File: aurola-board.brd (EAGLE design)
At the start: 86.4 x 31.8 mm, 84 parts, among them IC1 STM32F051C6T, J1 CONN_PWM, J2 CONN_TEMP, J3 CONN_FAN, J4 CONN_EC11, J5 CONN_I2C, P1 KF128-2P, Q1 600mA/40V, U1 ESP-01F, U2 BL9341, U3 BL9341

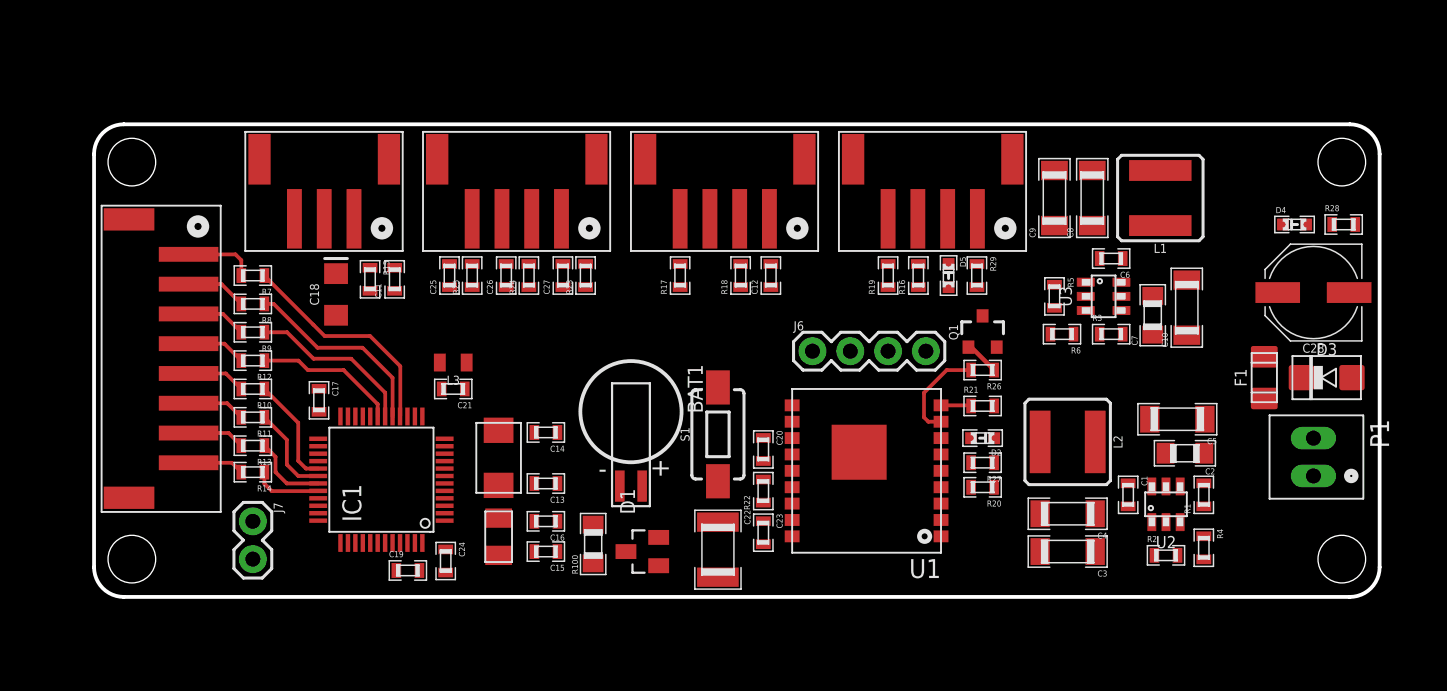
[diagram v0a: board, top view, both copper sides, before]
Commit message: 完成布局
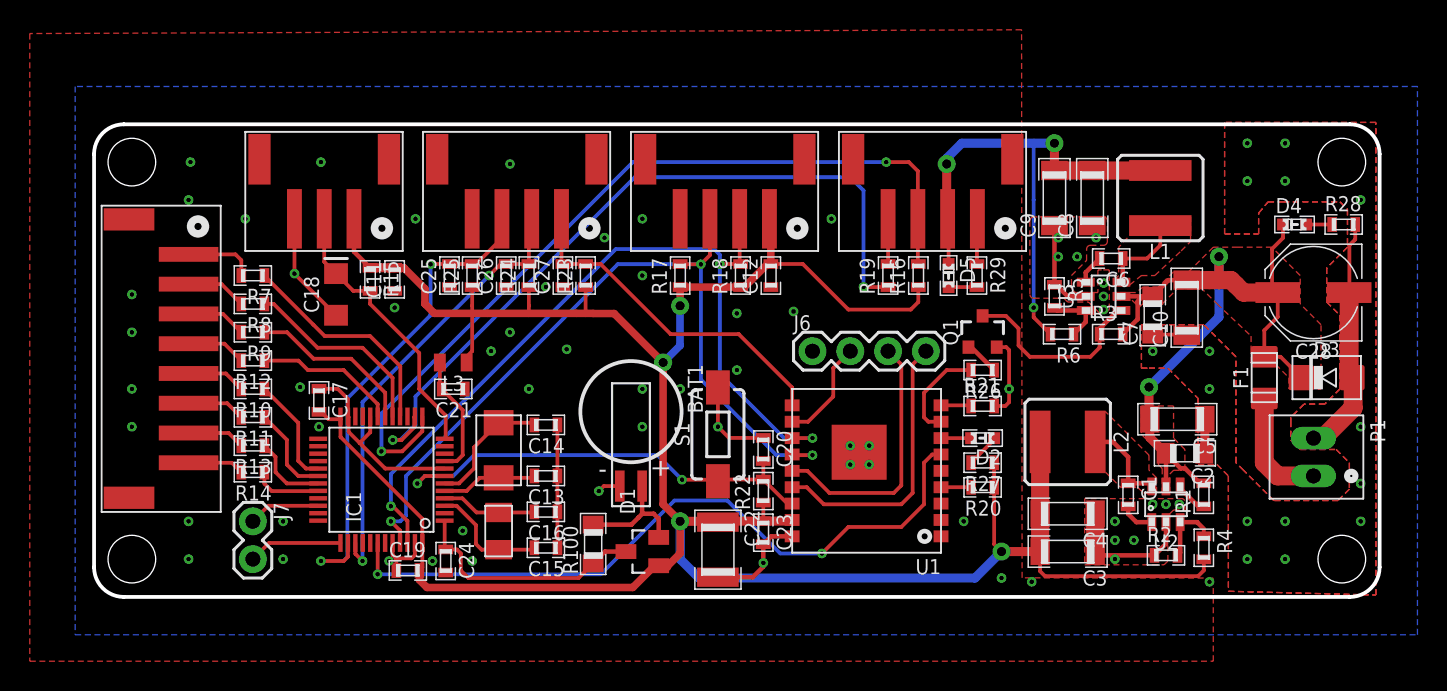
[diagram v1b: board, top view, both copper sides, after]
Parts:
- moved C16 0.63 mm to (30.4, 5.71)
- moved C14 0.51 mm to (30.4, 11.6)
- moved C13 0.51 mm to (30.4, 8.13)
- moved U$1 0.51 mm to (27.2, 8.00)
- moved U$2 0.38 mm to (27.2, 3.17)
- moved C15 0.25 mm to (30.4, 3.30)
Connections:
- removed net N$26: C28.+, D3.C, D4.P$1, F1.1
- new net EC_INT: IC1.42, U1.6
- net FAN_SPEED: now also IC1.13
- net VIN: now also C28.+, D3.C, D4.P$1, F1.1
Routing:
- net 3.3V: track 0.00 -> 173.9 mm, vias 0 -> 4
- net GND: track 0.00 -> 94.0 mm, vias 0 -> 78
- net FAN_SPEED: track 0.00 -> 56.4 mm, vias 0 -> 2
- net SDA: track 0.00 -> 55.6 mm, vias 0 -> 3
- net SCL: track 0.00 -> 54.7 mm, vias 0 -> 3
- net FAN_PWM: track 0.00 -> 51.1 mm, vias 0 -> 2
- net VIN: track 0.00 -> 50.7 mm, vias 0 -> 2
- net EC_INT: track 0.00 -> 47.9 mm, vias 0 -> 2
- net 12V: track 0.00 -> 37.1 mm, vias 0 -> 3
- net EC_A: track 0.00 -> 33.6 mm, vias 0 -> 2
- net RST: track 0.00 -> 30.7 mm, vias 0 -> 2
- net EC_B: track 0.00 -> 30.2 mm, vias 0 -> 2
- net EC_SW: track 0.00 -> 23.1 mm
- net TEMP_DO: track 0.00 -> 18.8 mm
- net TX: track 0.00 -> 18.8 mm
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- added copper zone on layer 1, net GND
- added copper zone on layer 16, net GND
- added copper zone on layer 1, net N$2
- added copper zone on layer 1, net N$6
- added copper zone on layer 1, net VIN
